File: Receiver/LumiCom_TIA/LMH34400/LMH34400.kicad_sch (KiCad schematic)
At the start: 24 parts, among them J1 TEST, J2 Conn_Coaxial, J3 Vout, J4 N_EN, J5 N_ALC, J6 Conn_Coaxial, U1 XLMH34400IDRLR

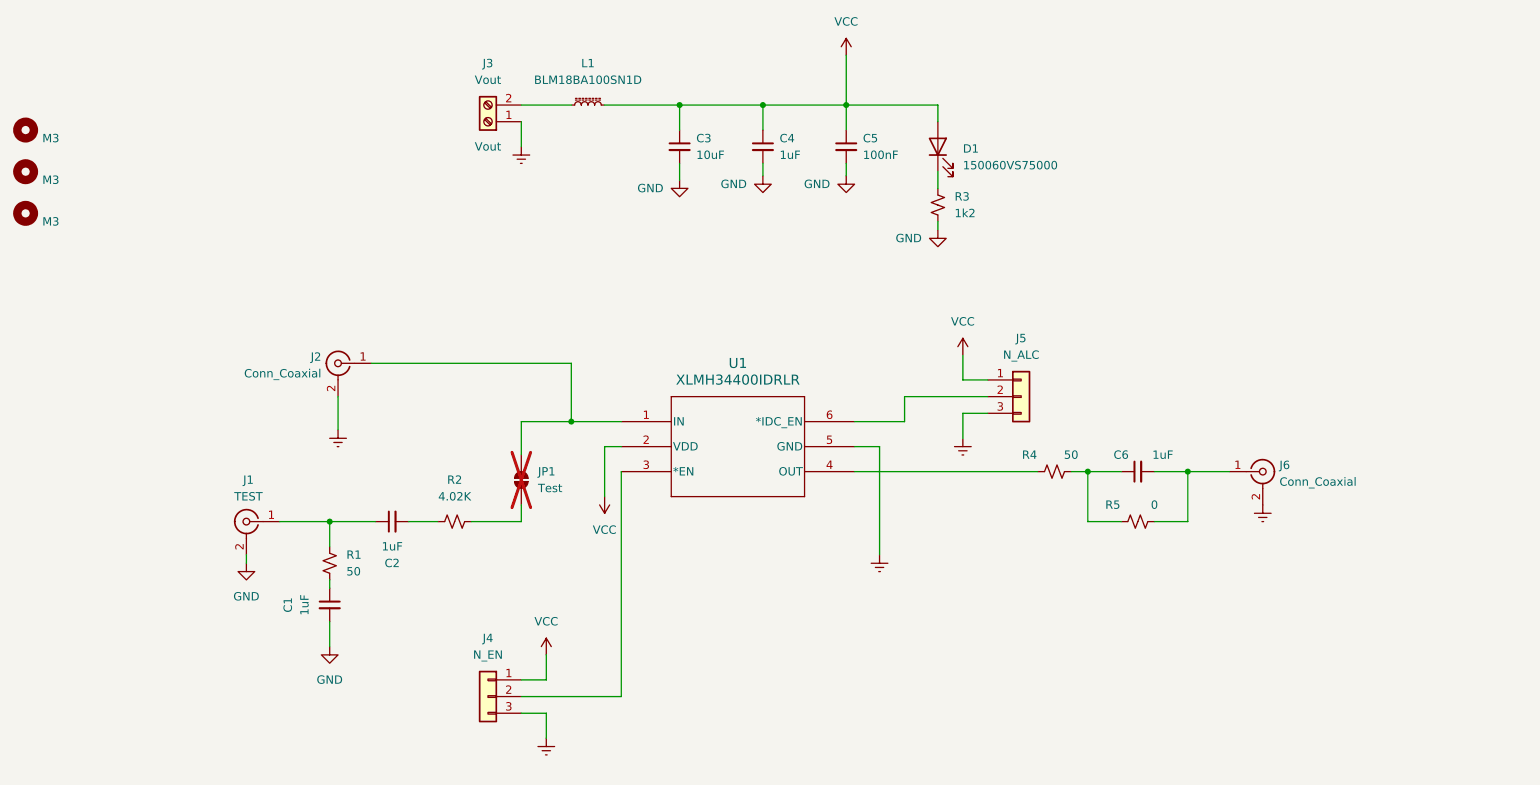
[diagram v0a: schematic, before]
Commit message: Small updates
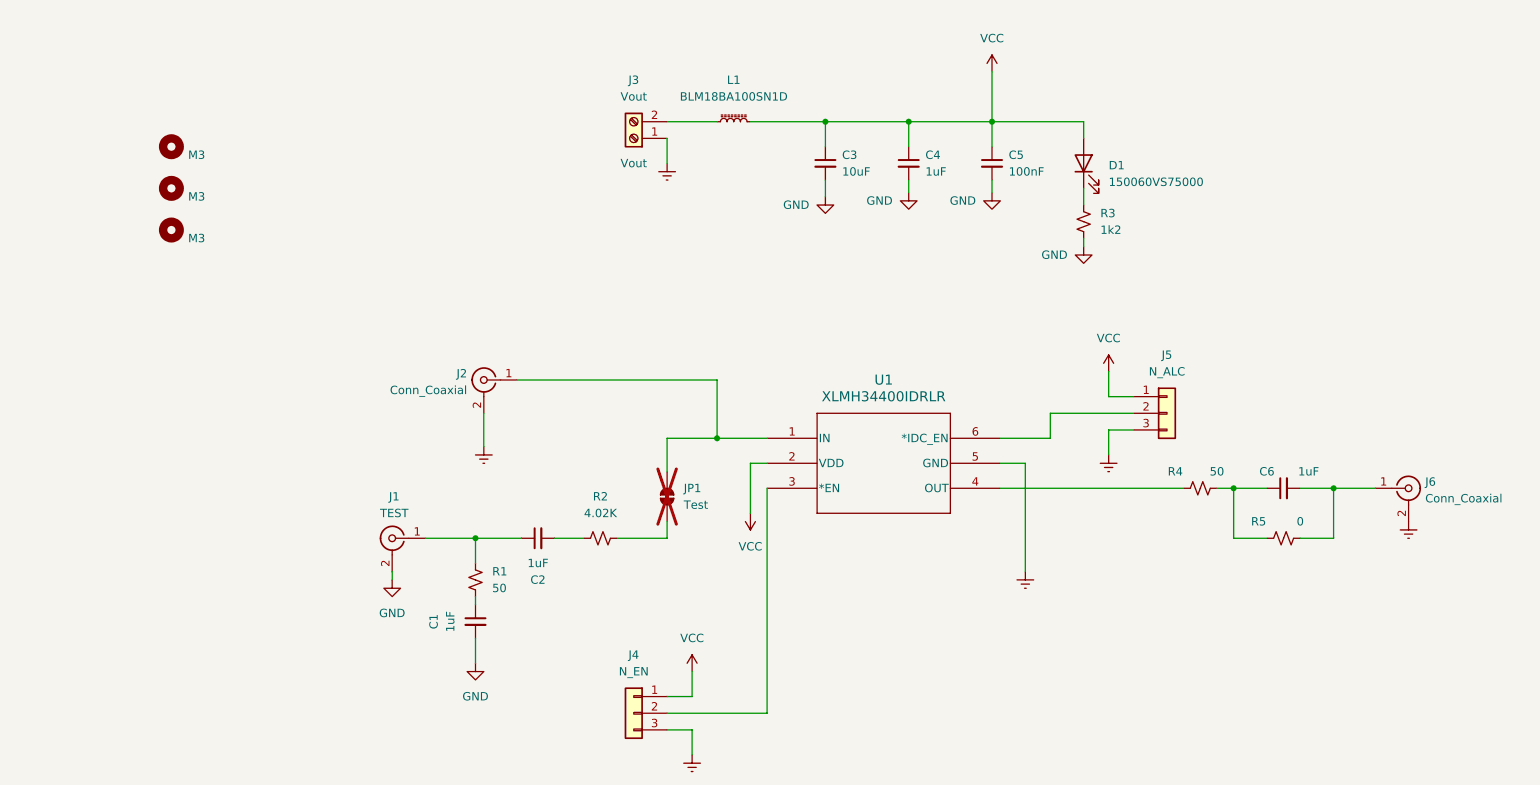
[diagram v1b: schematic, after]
